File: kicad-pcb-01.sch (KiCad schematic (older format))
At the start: 5 parts

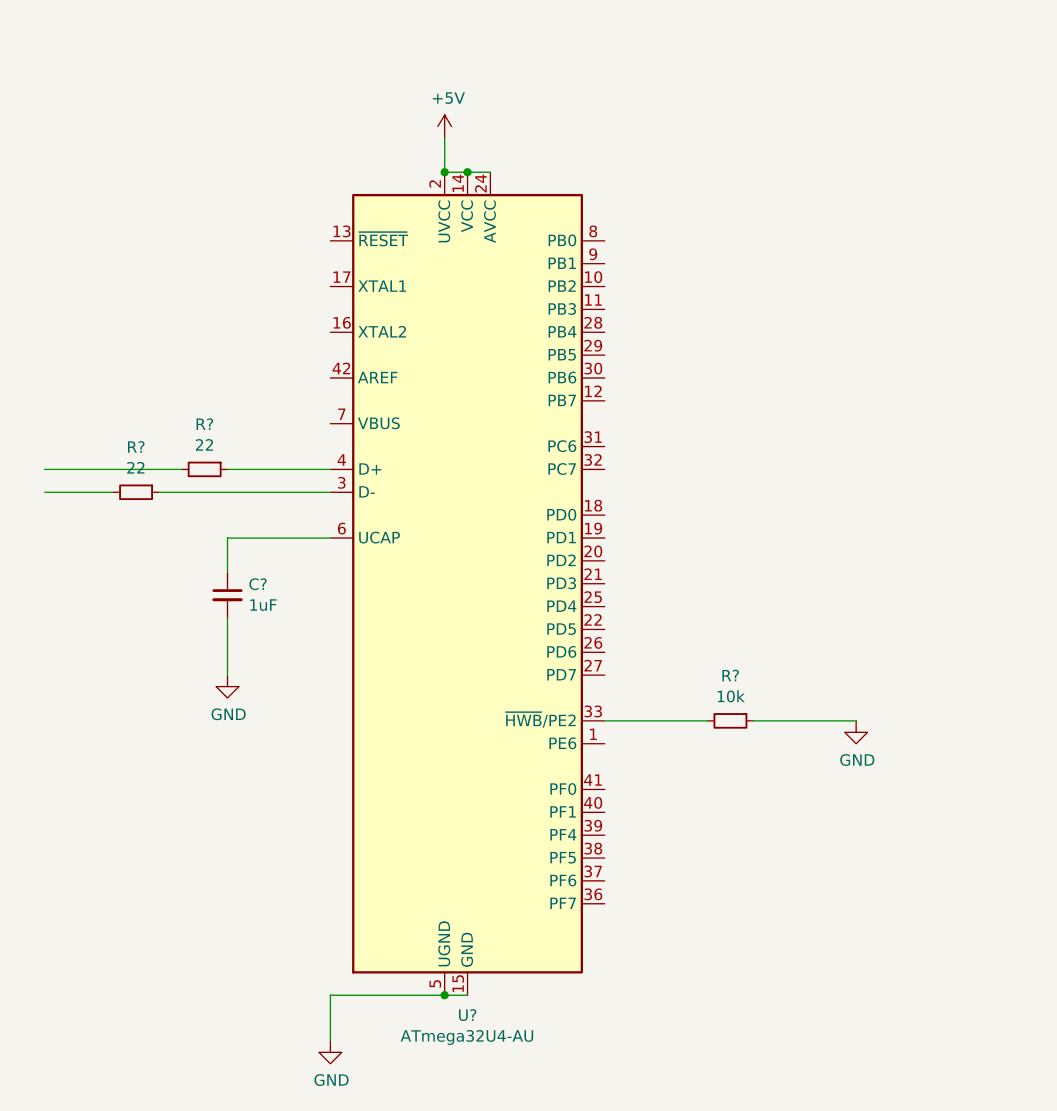
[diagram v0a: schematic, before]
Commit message: mcu ready part 3
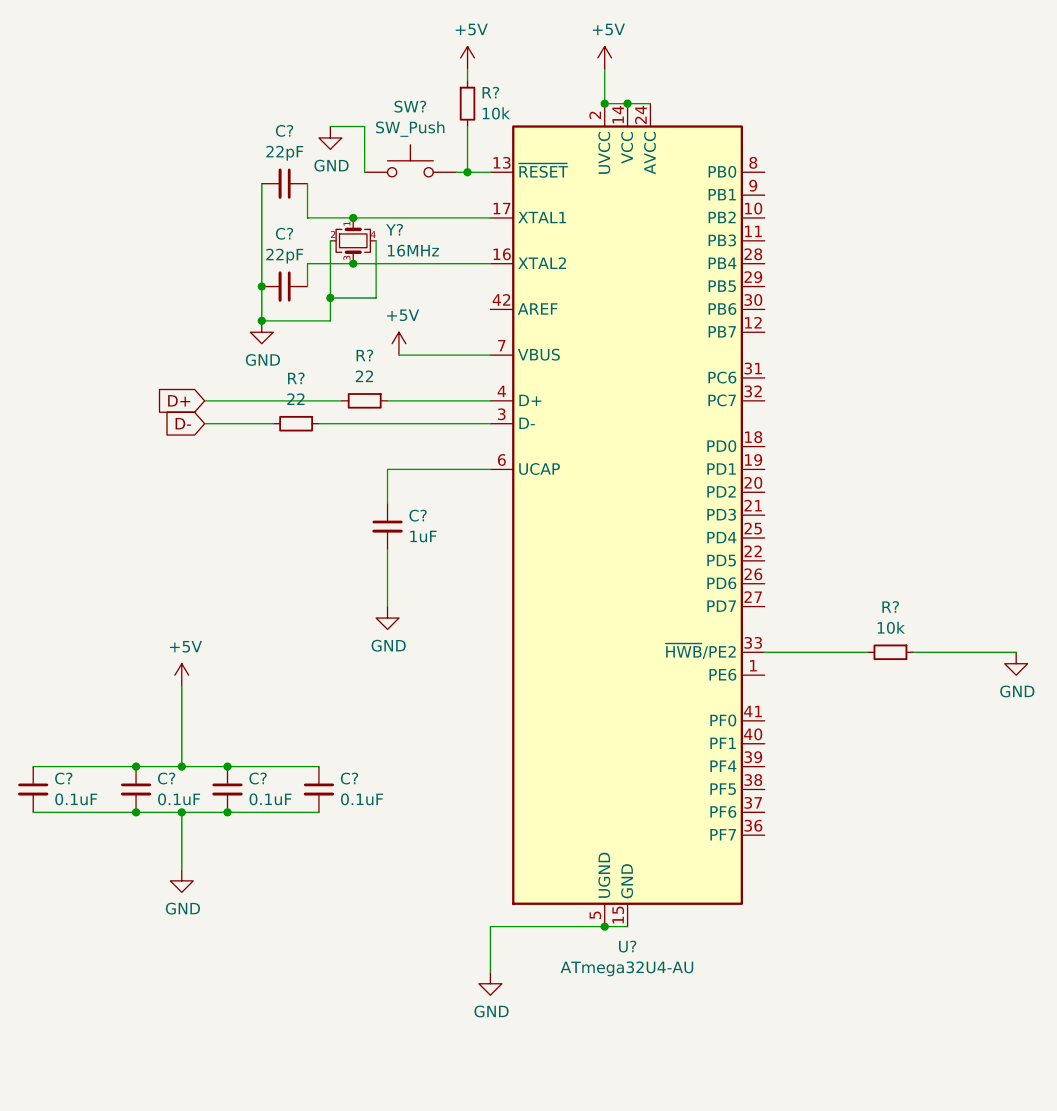
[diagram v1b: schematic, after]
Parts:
- added C? (x4): 0.1uF, symbol Device:C_Small
- added C? (x2): 22pF, symbol Device:C_Small
- added R?: 10k, symbol Device:R_Small
- added SW?: SW_Push, symbol Switch:SW_Push
- added Y?: 16MHz, symbol Device:Crystal_GND24_Small
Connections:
- net labels added: D+, D-
- wire segments 15 -> 45
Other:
- moved on the sheet: C?, R?, U?
